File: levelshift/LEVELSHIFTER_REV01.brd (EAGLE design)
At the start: 40.5 x 35 mm, 52 parts, among them IC1 3.3V, U1 SN6501DBVR, U2 TI-INA226

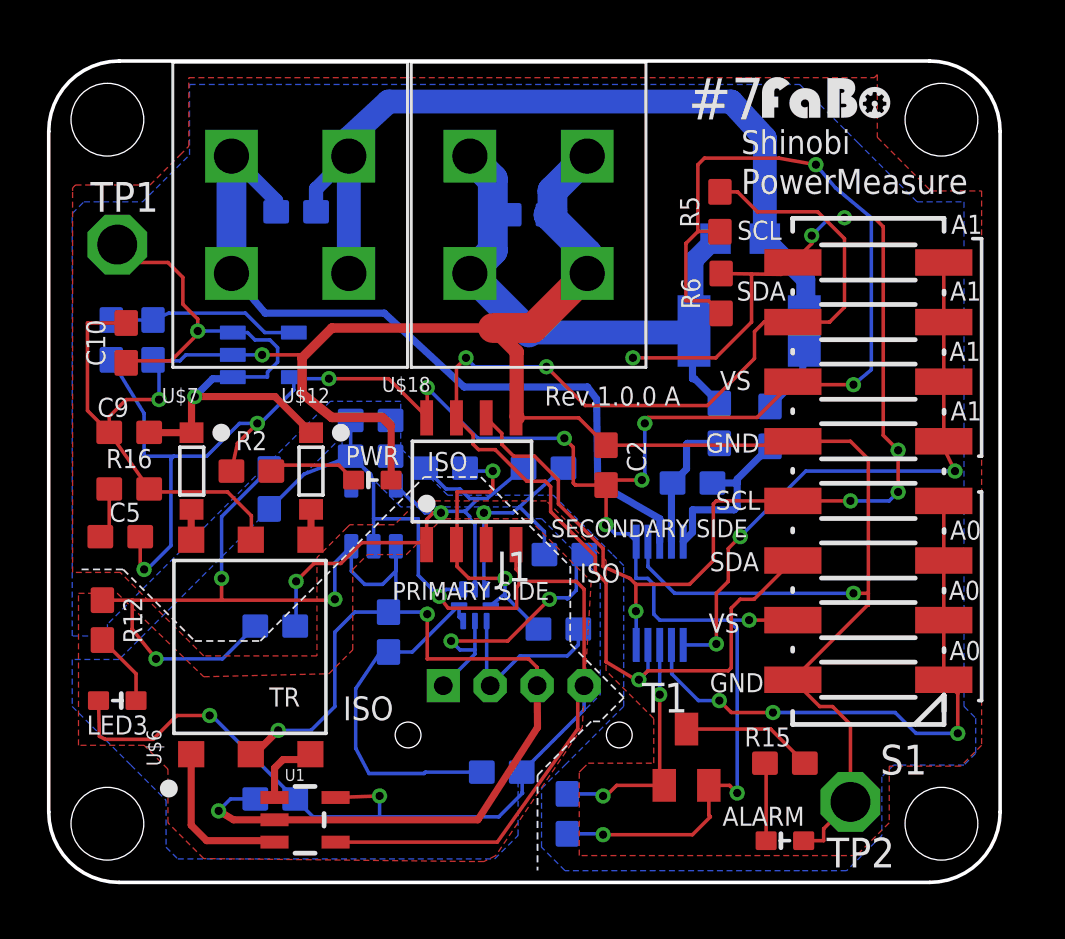
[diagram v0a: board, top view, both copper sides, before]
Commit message: LEVEL SHIFT NEW RELESE ADDTION.
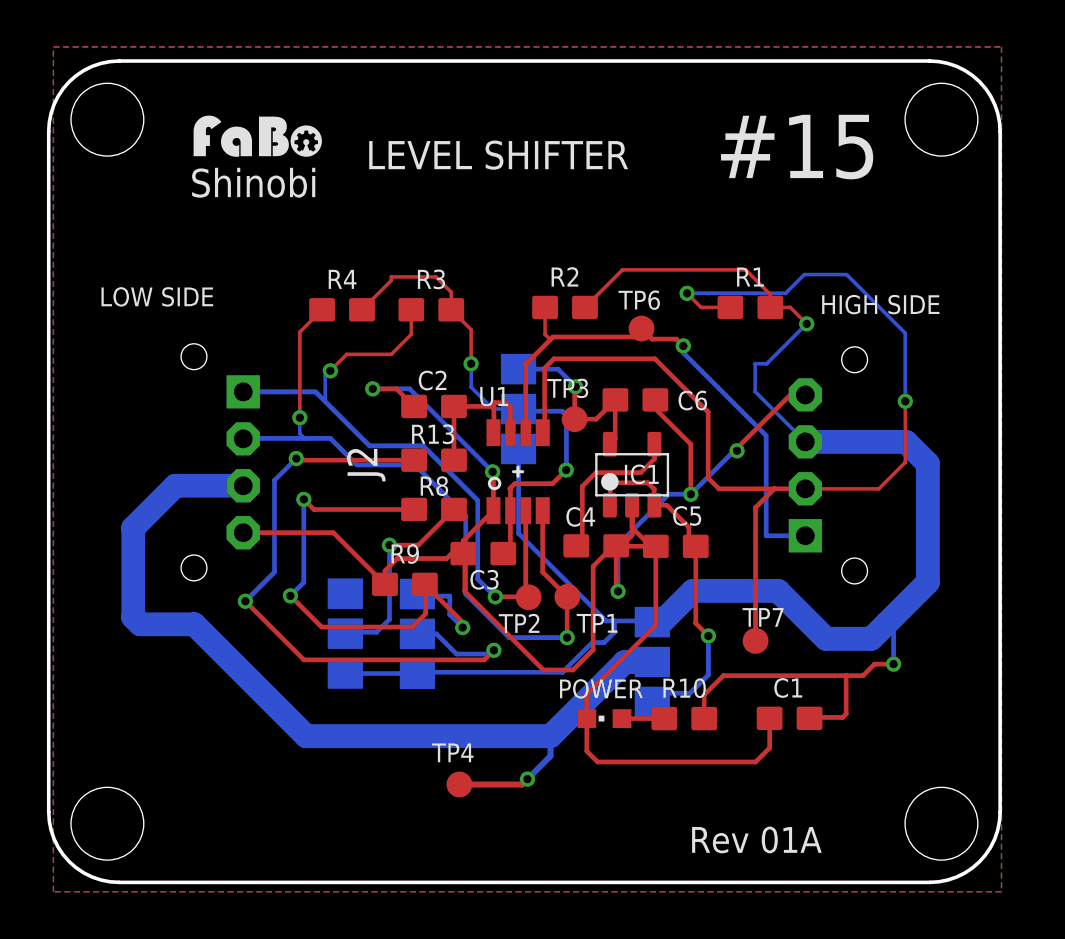
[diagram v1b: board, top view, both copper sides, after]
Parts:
- removed ALARM: RED, FaBo-LED:0603
- removed C10: 0.1uF, FaBo-Capacitor:0603
- removed C7: NC, FaBo-Capacitor:0603
- removed C8, C9: 10uF, FaBo-Capacitor:0603
- removed IC2: (no value), FaBo-LevelTranslator:XQFN8
- removed LED3: BLUE, FaBo-LED:0603
- removed PWR: GREEN, FaBo-LED:0603
- removed R11: 0Ω, FaBo-Resistors:0603
- removed R12: 1KΩ, FaBo-Resistors:0603
- removed R14, R5, R6: 4.7KΩ, FaBo-Resistors:0603
- removed R15: 510Ω, FaBo-Resistors:0603
- removed R16: 1Ω, FaBo-Resistors:0603
- removed R17, R18, R19: NC, FaBo-Resistors:0603
- removed R7: 10Ω, FaBo-Resistors:0603
- removed S1: 219-08J, switch-dil:CTS-219-08J
- removed SHUNT1: PMR10EZPFV2L00, FaBo:PMR10EZPFV2L00
- removed SHUNT2: WSL2010R0250FEB, FaBo:WSL2010R0250FEB
- removed T1: (no value), transistor:SC59-BEC
- removed U$12, U$7: MBR0520L, FaBo:MBR0502L
- removed U$18: ISO1541, FaBo:ISO1541
- removed U$19: (no value), FaBo-Logo:LOGO_FABO_S
- removed U$3: ML-1400-S1, FaBo-Terminal:ML-1400-S1
- removed U$5: (no value), FaBo-Template:FABO-SHINOBI
- removed U$6: 760390014, FaBo:760390014
- removed U$8: TPS76333, FaBo:TPS76333
- removed U2: TI-INA226, FaBo-Sensor:TI-INA226
- added J2: (no value), FaBo-Template 2:FABO_BRICK_I2C_S04B-PASK-2
- added JMP1, JMP2, JMP3, JMP4: 0R-JUMPA, jump-0r-smd:A0R-JMP
- added POWER: (no value), led:CHIPLED_0603
- added TP3, TP4, TP6, TP7: TPTP11R, testpad:TP11R
- added U$1: (no value), FaBo-Logo:LOGO_FABO_S
- C1: value 0.1uF -> 1uf
- C2, C3: value 0.1uF -> 0.1uf
- C4: value 0.1uF -> 0.01uf
- C5: value 10uF -> 1uf
- C6: value 1uF -> 2.2uf
- IC1: value 3.3V -> (none)
- J1: device FaBo-Template:FABO_BRICK_I2C_S04B-PASK-2 -> FaBo-Template 2:FABO_BRICK_I2C_S04B-PASK-2
- R1: value 4.7KΩ -> 4.7K
- R10: value 0Ω -> 1K
- R13: value 4.7KΩ -> 200K
- R2: value 1KΩ -> 4.7K
- R3: value 300K -> DNP
- R4: value 150K -> DNP
- R8: value 10Ω -> DNP
- R9: value 200KΩ -> DNP
- TP1, TP2: value TPPAD1-17 -> TPTP11R; device testpad:P1-17 -> testpad:TP11R
- U$2: value ML-1400-S1 -> (none); device FaBo-Terminal:ML-1400-S1 -> FaBo-Template 2:FABO-SHINOBI
- U1: value SN6501DBVR -> PCA9306DP1; device TI:SOT-23-5 -> FaBo-LevelTranslator:TSSOP8
- moved U$2 30.3 mm to (0.00, 0.00)
- moved R10 27.2 mm to (27.1, 6.98), flipped to the top, turned to 0 degrees
- moved TP1 24.4 mm to (22.1, 12.2)
- moved C5 23.7 mm to (26.7, 14.3)
- moved R1 22.9 mm to (29.9, 24.5), flipped to the top, turned to 0 degrees
- moved U1 17.4 mm to (20.0, 17.5)
- moved TP2 16.3 mm to (20.4, 12.2)
- moved J1 15.6 mm to (32.2, 17.8), turned to 270 degrees
- moved R2 15.1 mm to (22.0, 24.5)
- moved R3 13.7 mm to (16.3, 24.4), flipped to the top, turned to 0 degrees
- moved R8 12.7 mm to (16.4, 15.9), flipped to the top, turned to 0 degrees
- moved C6 11.5 mm to (25.0, 20.6), flipped to the top, turned to 180 degrees
- moved IC1 11.2 mm to (24.9, 17.4), flipped to the top
- moved C1 10.8 mm to (31.6, 6.99), flipped to the top, turned to 0 degrees
- moved C4 10.4 mm to (23.3, 14.3), flipped to the top, turned to 180 degrees
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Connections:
- removed net 3.3V: C2.2, C5.2, R1.2, R2.1, R3.2, R5.1, R6.1, S1.11, S1.15, T1.E, U$18.VCC2, U$8.OUT, U2.6
- removed net A0: S1.1, S1.2, S1.3, S1.4, U2.2
- removed net A1: S1.5, S1.6, S1.7, S1.8, U2.1
- removed net GND_SECONDARY: ALARM.CATHODE, C10.2, C2.1, C9.2, PWR.CATHODE, R11.2, R16.2, R4.2, S1.12, S1.16, TP2.TP, U$18.GND2, U$3.RIGHT1, U$3.RIGHT2, U$6.5, U$8.GND, U2.7
- removed net N$11: IC2.4, R14.1, R18.2, U$18.SDA1
- removed net N$12: IC2.6, J1.SCL, R17.1
- removed net N$14: U$12.P$2, U$6.4
- removed net N$16: C10.1, C9.1, TP1.TP, U$12.P$1, U$7.P$1, U$8.EN, U$8.IN
- removed net N$22: IC2.5, J1.SDA, R18.1
- removed net N$23: IC2.3, R13.1, R17.2, U$18.SCL1
- removed net N$5: R1.1, T1.B, U2.3
- removed net N$6: U$6.6, U$7.P$2
- removed net SCL: R6.2, S1.13, S1.9, U$18.SCL2, U2.5
- removed net SDA: R5.2, S1.10, S1.14, U$18.SDA2, U2.4
- removed net VBUS: R10.1, U$2.LEFT1, U$2.LEFT2, U2.8
- removed net VIN+: R10.2, R7.2, SHUNT1.P$2, SHUNT2.P$2, U$2.RIGHT1, U$2.RIGHT2
- removed net VIN-: R11.1, R8.2, SHUNT1.P$1, SHUNT2.P$1, U$3.LEFT1, U$3.LEFT2
- new net N$27: POWER.A, R10.1
- new net VCC: C1.2, J1.VCC, JMP1.3, JMP2.1, JMP3.1, JMP4.3, R1.2, R10.2, R2.2
- net GND: now also C1.1, C2.1, C5.1, C6.1, J2.GND, POWER.C, R9.1, U1.GND; no longer C6.2, C7.2, C8.1, IC2.1, LED3.CATHODE, U$18.GND1, U1.4, U1.5
- net N$1: now also J1.SDA, R1.1, TP7.TP, U1.SDA2; no longer C1.2, R7.1, U2.10
- net N$10: now also C5.2, IC1.1, IC1.3, JMP2.3; no longer LED3.ANODE, R12.2
- net N$13: now also JMP4.2, R8.2; no longer C6.1, C7.1, IC1.5, IC2.2, R13.2, R14.2, R19.1, U$18.VCC1
- net N$18: now also C6.2, IC1.5, JMP1.1, TP3.TP; no longer C4.2, IC2.7, IC2.8, R9.2
- net N$19: now also JMP3.2, R13.1; no longer C3.2, C8.2, IC1.1, IC1.3, J1.VCC, R12.1, R19.2, R9.1, U$6.2, U1.2
- net N$2: now also J1.SCL, R2.1, TP6.TP, U1.SCL2; no longer C1.1, R8.1, U2.9
- net N$20: now also C4.2, IC1.4; no longer R3.1, R4.1, U$8.NC/FB
- net N$21: now also J2.VCC, JMP2.2, TP4.TP; no longer C5.1, R16.1
- net N$3: now also C2.2, R13.2, U1.EN, U1.VREF2; no longer U$6.1, U1.3
- net N$4: now also JMP3.3, R8.1, R9.2; no longer U$6.3, U1.1
- net N$7: now also J2.SCL, R3.1, TP2.TP, U1.SCL1; no longer ALARM.ANODE, R15.1
- net N$8: now also J2.SDA, R4.1, TP1.TP, U1.SDA1; no longer PWR.ANODE, R2.2
- net N$9: now also C3.2, JMP1.2, R3.2, R4.2, U1.VREF1; no longer R15.2, T1.C
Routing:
- net 3.3V: track 108.0 -> 0.00 mm, vias 13 -> 0
- net GND_SECONDARY: track 106.9 -> 0.00 mm, vias 3 -> 0
- net VCC: track 0.00 -> 81.6 mm, vias 0 -> 2
- net SDA: track 59.5 -> 0.00 mm, vias 3 -> 0
- net SCL: track 54.9 -> 0.00 mm, vias 7 -> 0
- net N$19: track 72.9 -> 27.5 mm, vias 6 -> 3
- net VIN+: track 40.6 -> 0.00 mm
- net N$1: track 8.05 -> 47.8 mm, vias 0 -> 2
- net N$21: track 2.19 -> 40.0 mm, vias 0 -> 1
- net VBUS: track 33.5 -> 0.00 mm
- net VIN-: track 27.5 -> 0.00 mm
- net N$16: track 27.5 -> 0.00 mm, vias 2 -> 0
- net N$8: track 3.83 -> 31.1 mm, vias 0 -> 2
- net A1: track 25.7 -> 0.00 mm, vias 3 -> 0
- net N$7: track 3.32 -> 28.0 mm, vias 0 -> 2
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- removed copper zone on layer 1, net GND_SECONDARY
- removed copper zone on layer 16, net GND_SECONDARY
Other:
- board text added: "#15"
- board text added: "HIGH SIDE"
- board text added: "LEVEL SHIFTER"
- board text added: "LOW SIDE"
- board text added: "Rev 01A"
- board text removed: "#7"
- board text removed: "0x40 0x41 0x42 0x43 0x44 0x45 0x46 0x47"
- board text removed: "A0"
- board text removed: "A0 | A1 | ADDRESS GND GND GND VS GND SDA GND SCL VS GND VS VS VS SDA VS SCL"
- board text removed: "A1"
- board text removed: "GND"
- board text removed: "IN+"
- board text removed: "IN-"
- board text removed: "ISO"
- board text removed: "PRIMARY SIDE"
- board text removed: "PowerMeasure"
- board text removed: "Rev.1.0.0 A"
- board text removed: "S-PM01"
- board text removed: "SCL"
- board text removed: "SDA"
- board text removed: "SECONDARY SIDE"
- board text removed: "TR"
- board text removed: "VBUS"
- board text removed: "VS"
